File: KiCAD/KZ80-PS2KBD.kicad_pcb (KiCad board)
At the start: 2 copper layers, 100 x 75 mm, 23 parts, among them J1 232C(DEBUG), J2 PS/2 KB, J3 SBC8080 BUS, J4 ADR-JP2, J5 ADR-JP1, J6 ICSP, J7 CON-A, U1 74HC139, U2 74HC00, U3 8255, U4 ATmega328P-PU

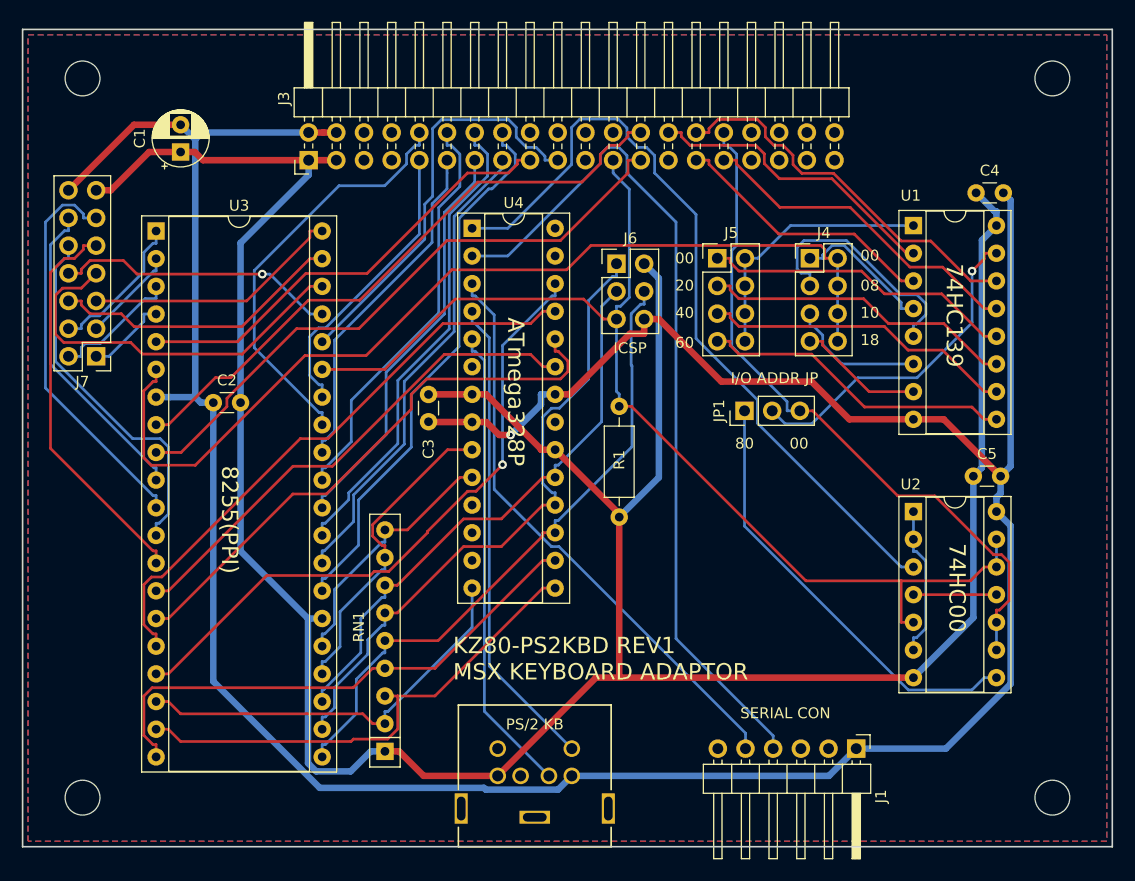
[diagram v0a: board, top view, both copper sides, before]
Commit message: REV1基板製造用ガーバーデータ出力版
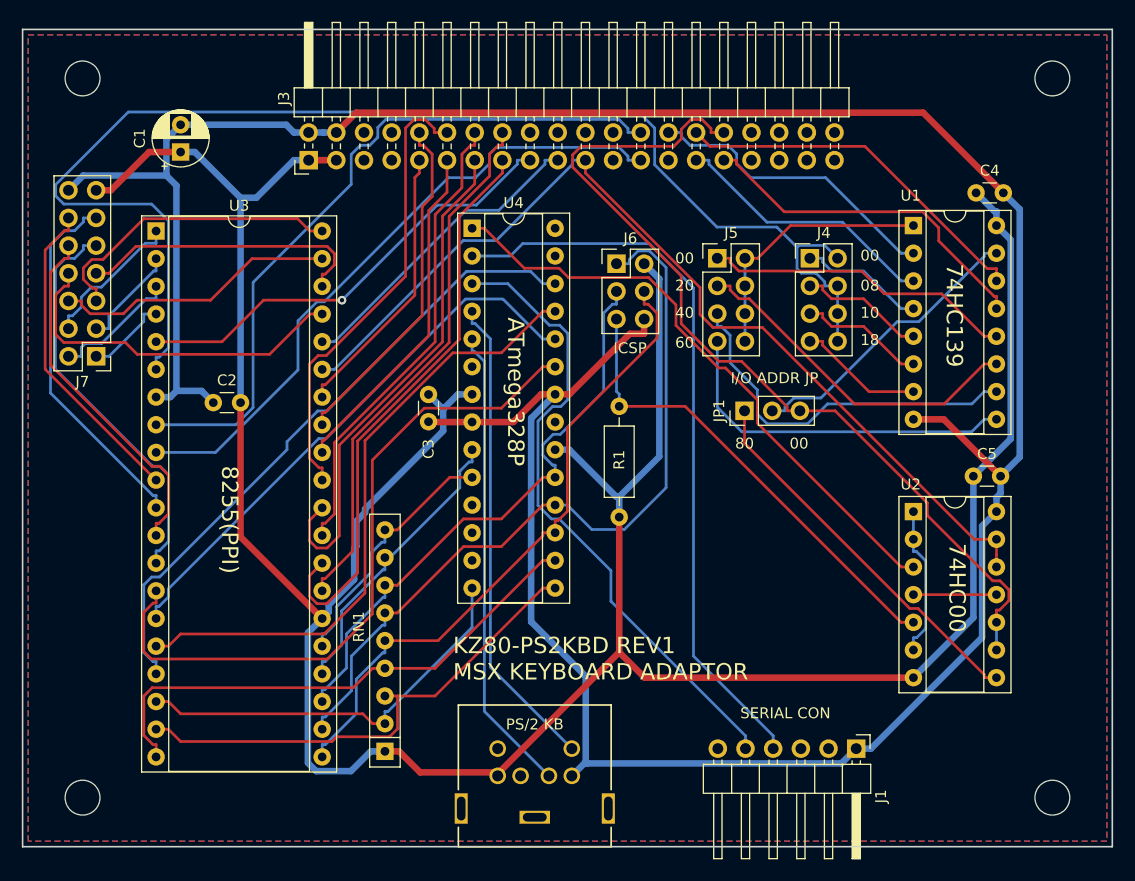
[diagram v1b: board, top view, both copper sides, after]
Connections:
- J1 pad 4: TxD -> RxD
- J1 pad 5: RxD -> TxD
- J3 pad 21: Net-(J3-Pad21) -> RESET
- J3 pad 23: RESET -> Net-(J3-Pad23)
- J6 pad 5: RESET -> /~RESET
- R1 pad 2: RESET -> /~RESET
- U2 pad 5: RESET -> /~RESET
- U4 pad 2: TxD -> RxD
- U4 pad 3: RxD -> TxD
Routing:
- net /~RESET: track 0.00 -> 43.3 mm
- net PPI-CE: track 89.6 -> 120.4 mm
- net TxD: track 79.1 -> 58.7 mm
- net /A7: track 63.4 -> 83.3 mm
- net Net-(U3-Pad14): track 46.1 -> 63.6 mm
- net Net-(U2-Pad3): track 73.0 -> 55.7 mm
- net RESET: track 103.7 -> 89.1 mm
- net RxD: track 53.6 -> 67.8 mm
- net /MISO: track 59.3 -> 71.9 mm
- net VCC: track 257.8 -> 269.4 mm
- net Net-(J4-Pad3): track 22.6 -> 11.6 mm
- net A1: track 56.3 -> 65.7 mm
- net /PA6: track 35.9 -> 26.8 mm
- net ~IOWR: track 37.9 -> 28.7 mm
- net /D6: track 43.9 -> 52.8 mm
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
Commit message: 74HC00 電源ピン配線見直しプリントパターン作成
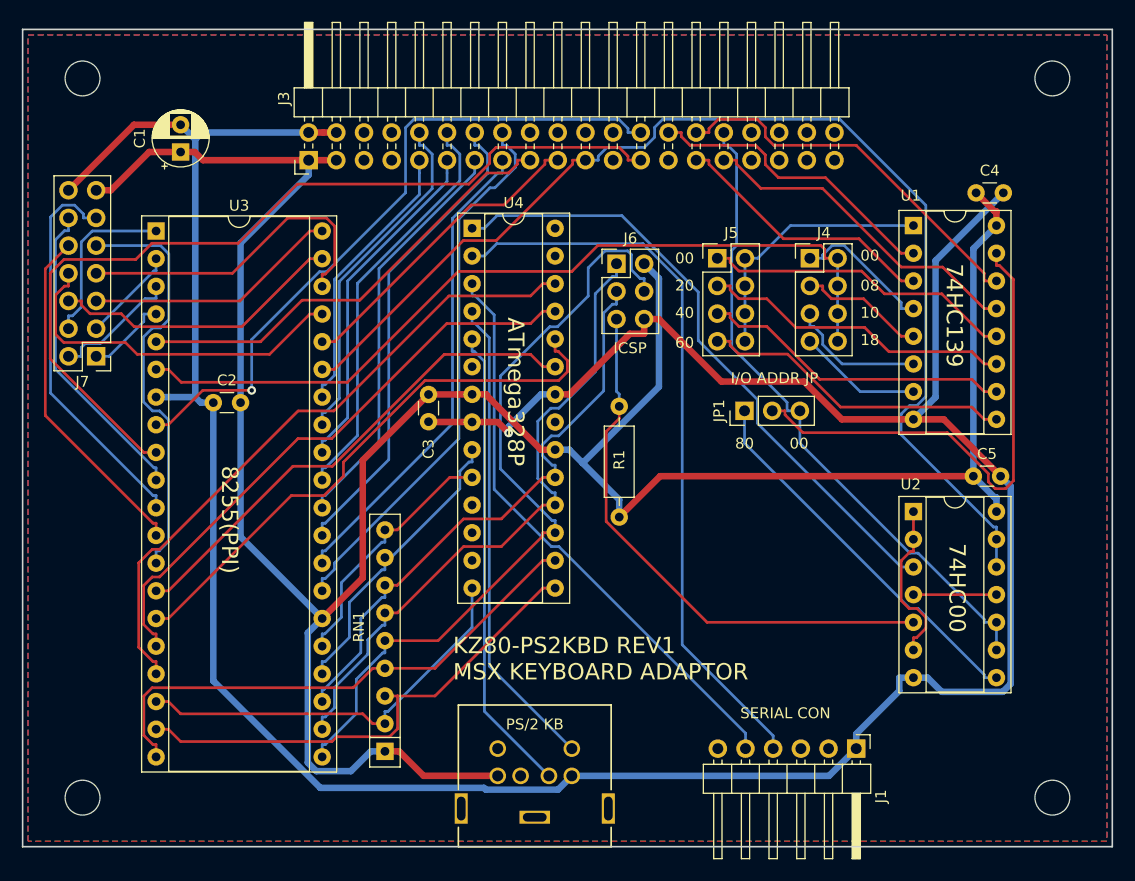
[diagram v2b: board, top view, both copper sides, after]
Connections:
- U2 pad 14: GND -> VCC
- U2 pad 7: VCC -> GND
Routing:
- net PPI-CE: track 120.4 -> 76.8 mm
- net VCC: track 269.4 -> 240.3 mm
- net /A7: track 83.3 -> 60.2 mm
- net A0: track 59.9 -> 81.3 mm
- net Net-(JP1-Pad2): track 26.9 -> 47.7 mm
- net RESET: track 89.1 -> 107.4 mm
- net Net-(U3-Pad14): track 63.6 -> 46.1 mm
- net /MOSI: track 60.1 -> 72.4 mm
- net /MISO: track 71.9 -> 59.7 mm
- net /D4: track 46.6 -> 37.9 mm
- net /D6: track 52.8 -> 44.2 mm
- net /~RESET: track 43.3 -> 51.2 mm
- net Net-(J5-Pad5): track 34.5 -> 28.8 mm
- net TxD: track 58.7 -> 53.6 mm
- net /PA4: track 28.0 -> 23.4 mm
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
